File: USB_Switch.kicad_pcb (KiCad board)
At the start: 2 copper layers, 53.3 x 25.4 mm, 18 parts, among them U1 AMS1117-3.3, U2 INA219AxD, U3 INA219AxD, U4 ESP-12F

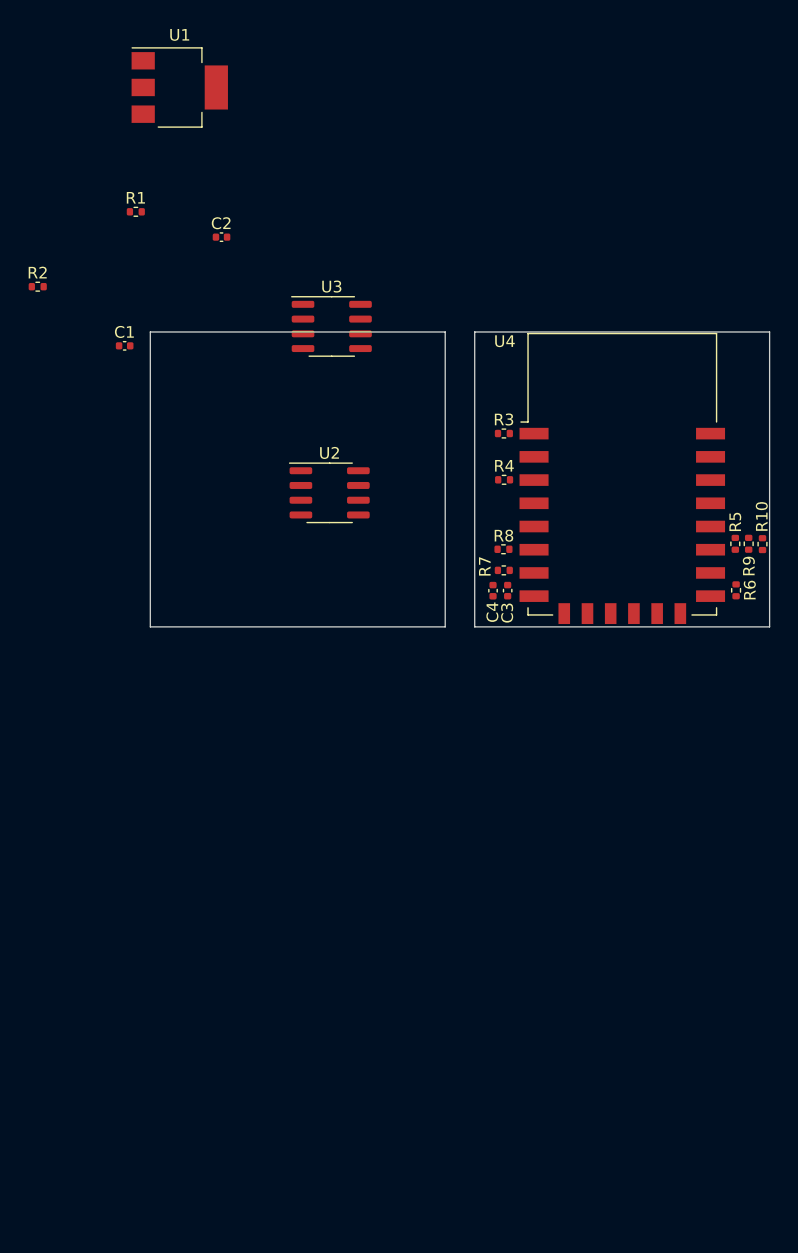
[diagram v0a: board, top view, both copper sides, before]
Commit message: Did work on schematic
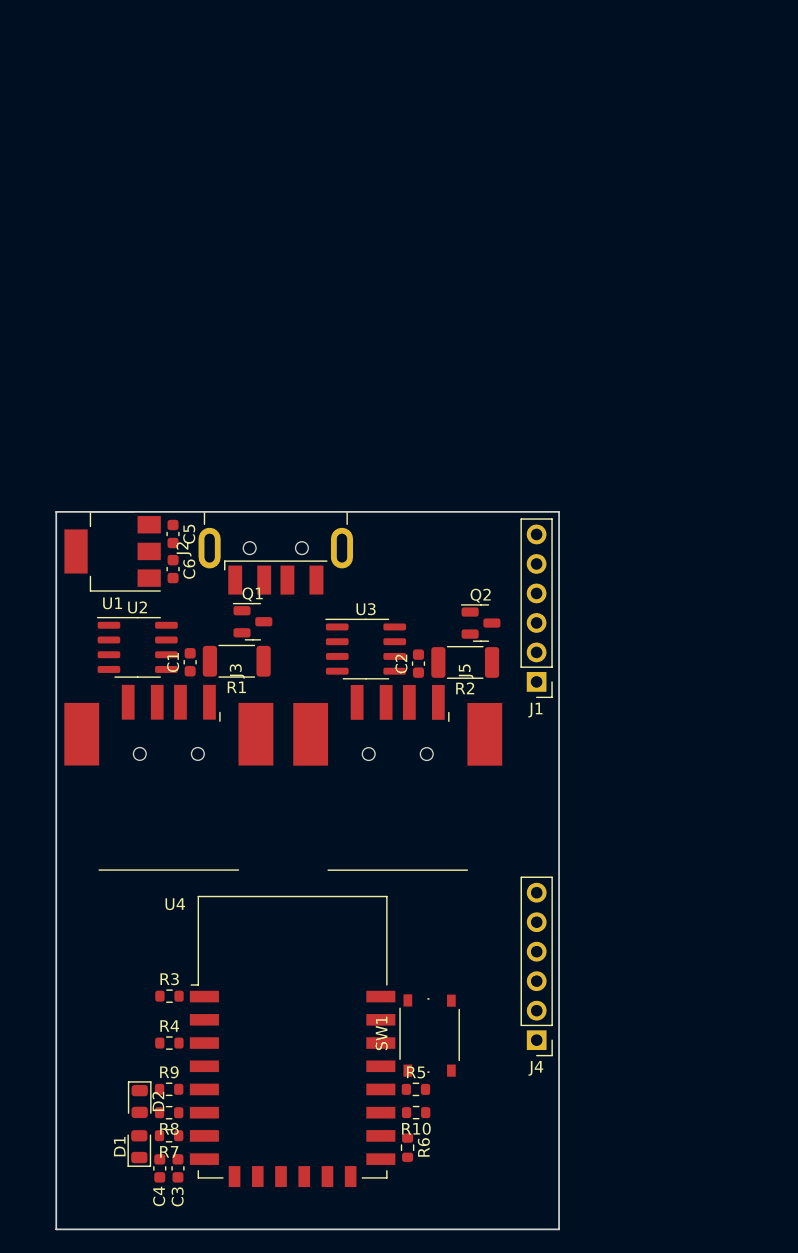
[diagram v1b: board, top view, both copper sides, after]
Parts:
- added C5: 10uF, Capacitor_SMD:C_0603_1608Metric, F.Cu at (45.1, 86.0)
- added C6: 10uF, Capacitor_SMD:C_0603_1608Metric, F.Cu at (45.1, 89.0)
- added D1: GREEN, LED_SMD:LED_0805_2012Metric, F.Cu at (42.2, 138.7)
- added D2: GREEN, LED_SMD:LED_0805_2012Metric, F.Cu at (42.3, 134.9)
- added J1: Conn_01x06, Connector_PinHeader_2.54mm:PinHeader_1x06_P2.54mm_Vertical, F.Cu at (76.4, 98.7)
- added J2: USB_IN, Library:U217-041N-4BV81, F.Cu at (54.0, 80.3)
- added J3: USB_OUT, Library:904-131A2032S10100, F.Cu at (44.8, 102.1)
- added J4: Conn_01x06, Connector_PinHeader_2.54mm:PinHeader_1x06_P2.54mm_Vertical, F.Cu at (76.5, 129.6)
- added J5: USB_OUT, Library:904-131A2032S10100, F.Cu at (64.5, 102.1)
- added Q1: Q_NMOS_GDS, Library:YJL3400A, F.Cu at (52.0, 93.5)
- added Q2: Q_NMOS_GDS, Library:YJL3400A, F.Cu at (71.7, 93.6)
- added SW1: PRGM, Library:TS-1187A-B-A-B, F.Cu at (67.1, 129.1)
- C1, C2, C3, C4: footprint Capacitor_SMD:C_0402_1005Metric -> Capacitor_SMD:C_0603_1608Metric
- R1, R2: footprint Resistor_SMD:R_0402_1005Metric -> Resistor_SMD:R_2010_5025Metric
- R10, R3, R4, R5, R6, R7, R8, R9: footprint Resistor_SMD:R_0402_1005Metric -> Resistor_SMD:R_0603_1608Metric
- moved R9 68.6 mm to (44.8, 133.8), turned to 0 degrees
- moved C4 57.4 mm to (44.0, 140.6), turned to -90 degrees
- moved R10 57.3 mm to (66.1, 135.8), turned to 180 degrees
- moved C3 57.3 mm to (45.6, 140.6), turned to -90 degrees
- moved R7 56.6 mm to (44.8, 137.8)
- moved R4 56.4 mm to (44.8, 129.8)
- moved R8 56.4 mm to (44.8, 135.8)
- moved R3 56.4 mm to (44.8, 125.8)
- moved U4 56.2 mm to (55.4, 129.3)
- moved R6 55.7 mm to (65.3, 138.8)
- moved R5 54.4 mm to (66.1, 133.8), turned to 0 degrees
- moved R2 49.0 mm to (70.3, 97.0), turned to 180 degrees
- moved C2 40.5 mm to (66.3, 97.1), turned to 90 degrees
- moved U1 40.4 mm to (39.9, 87.5), turned to 180 degrees
- moved R1 39.7 mm to (50.6, 96.9), turned to 180 degrees
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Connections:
- net /Control Board/C_GND renamed GND
- net /Control Board/LED_OFF renamed /Control Board/LED_2
- net /Control Board/LED_ON renamed /Control Board/LED_1
- C1 pad 1: /Control Board/C_3v3 -> /MOSFET Board/M_3v3
- C2 pad 1: /Control Board/C_3v3 -> /MOSFET Board/M_3v3
- R1 pad 2: /MOSFET Board/5V_OUT -> /MOSFET Board/5V_OUT_1
- R2 pad 2: /MOSFET Board/5V_OUT -> /MOSFET Board/5V_OUT_2
- U1 pad 2: /Control Board/C_3v3 -> /MOSFET Board/M_3v3
- U2 pad 3: /Control Board/C_I2C_SDA -> /MOSFET Board/M_I2C_SDA
- U2 pad 4: /Control Board/C_I2C_SCL -> /MOSFET Board/M_I2C_SCL
- U2 pad 5: /Control Board/C_3v3 -> /MOSFET Board/M_3v3
- U2 pad 7: /MOSFET Board/5V_OUT -> /MOSFET Board/5V_OUT_1
- U3 pad 2: /Control Board/C_3v3 -> /MOSFET Board/M_3v3
- U3 pad 3: /Control Board/C_I2C_SDA -> /MOSFET Board/M_I2C_SDA
- U3 pad 4: /Control Board/C_I2C_SCL -> /MOSFET Board/M_I2C_SCL
- U3 pad 5: /Control Board/C_3v3 -> /MOSFET Board/M_3v3
- U3 pad 7: /MOSFET Board/5V_OUT -> /MOSFET Board/5V_OUT_2
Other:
- board size 53.3 x 25.4 mm -> 43.3 x 61.8 mm
- board text added: "V-CUT"
